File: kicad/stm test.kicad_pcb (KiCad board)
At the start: 2 copper layers, 2 parts, among them U101 MCP23008-xP

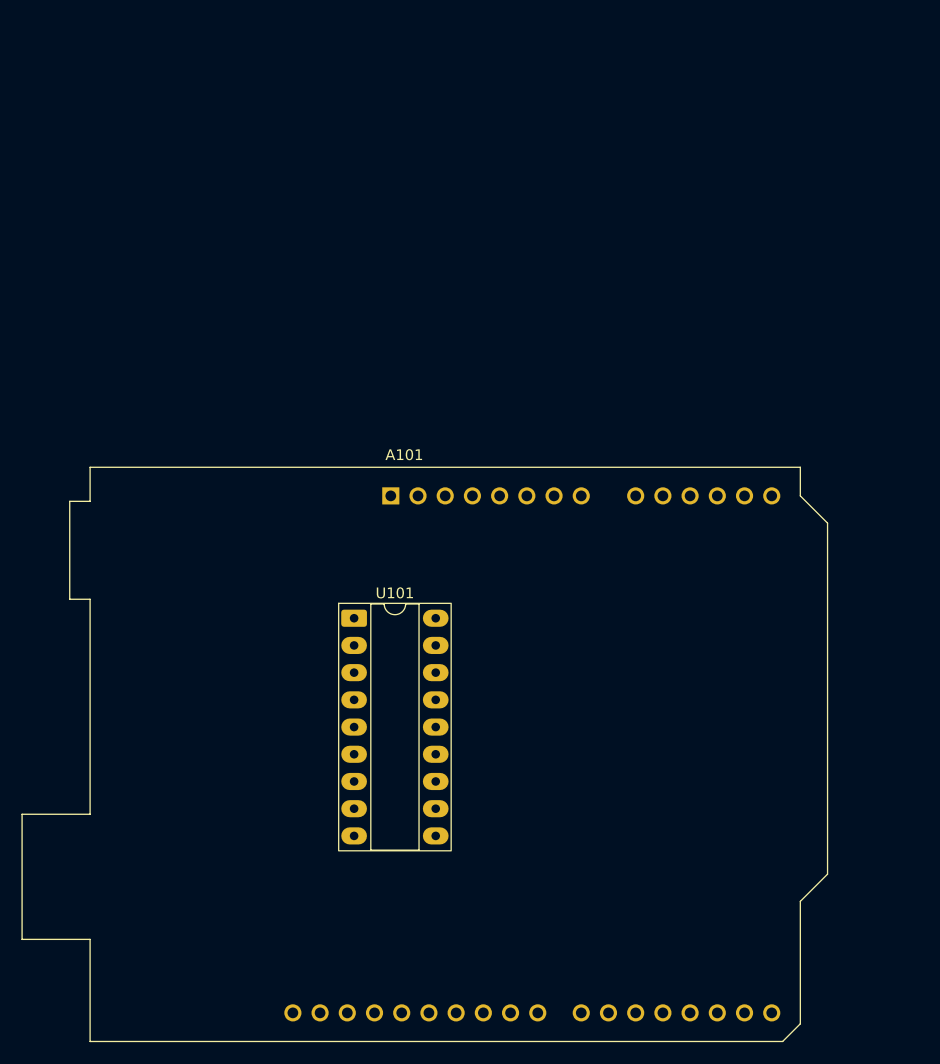
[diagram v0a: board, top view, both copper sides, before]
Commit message: i fugged up
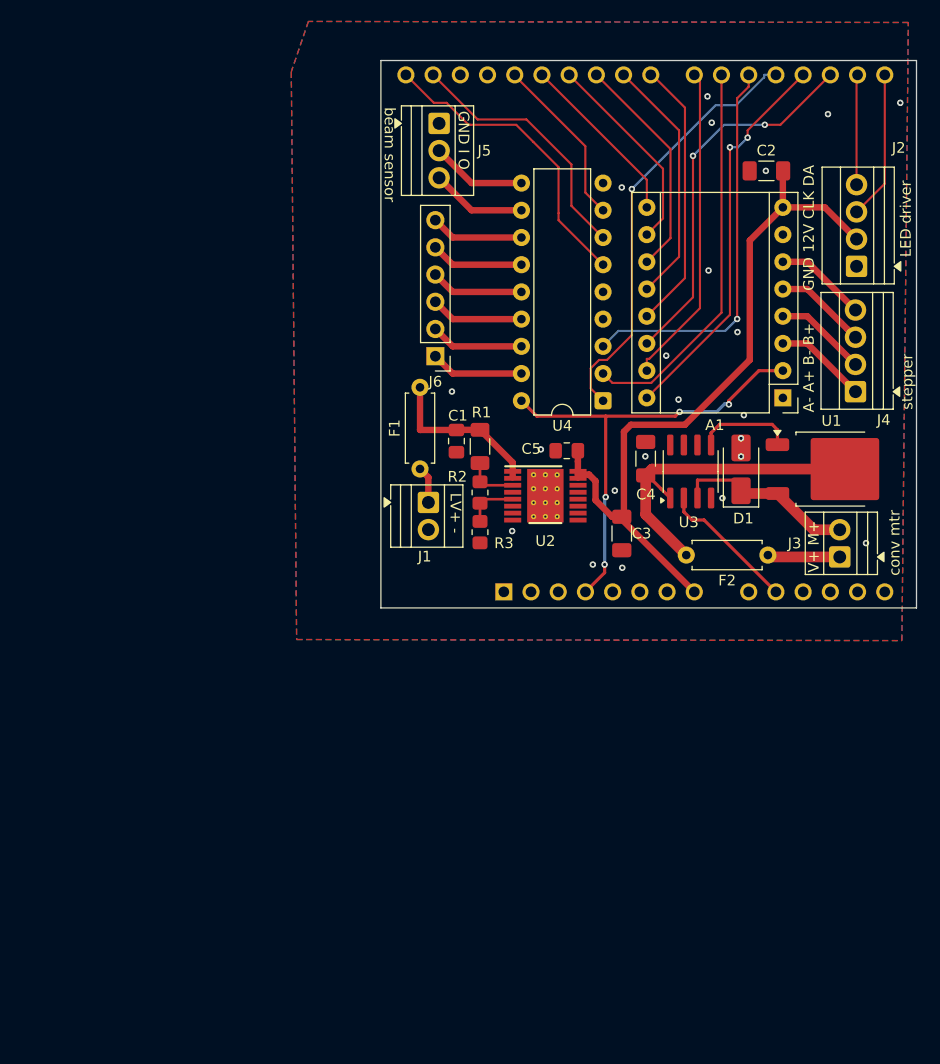
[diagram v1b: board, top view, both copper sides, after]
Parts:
- removed A101: Arduino_UNO_R3, Module:Arduino_UNO_R3
- removed U101: MCP23008-xP, Package_DIP:DIP-18_W7.62mm_Socket_LongPads
- added A1: Pololu_Breakout_A4988, Module:Pololu_Breakout-16_15.2x20.3mm, F.Cu at (158.0, 86.0)
- added A2: Arduino_UNO_R3, Module:Arduino_UNO_R3, B.Cu at (132.0, 104.1)
- added C1: 220n, Capacitor_SMD:C_0805_2012Metric_Pad1.18x1.45mm_HandSolder, F.Cu at (127.6, 90.0)
- added C2: 10u, Capacitor_SMD:C_1206_3216Metric_Pad1.33x1.80mm_HandSolder, F.Cu at (156.5, 64.8)
- added C3: 10u, Capacitor_SMD:C_1206_3216Metric_Pad1.33x1.80mm_HandSolder, F.Cu at (143.0, 98.7)
- added C4: 10u, Capacitor_SMD:C_1206_3216Metric_Pad1.33x1.80mm_HandSolder, F.Cu at (145.2, 91.7)
- added C5: 220n, Capacitor_SMD:C_0805_2012Metric_Pad1.18x1.45mm_HandSolder, F.Cu at (137.9, 90.9)
- added D1: ES1D, Diode_SMD:D_SMA, F.Cu at (154.1, 92.7)
- added F1: 1.5A, Resistor_THT:R_Axial_DIN0207_L6.3mm_D2.5mm_P7.62mm_Horizontal, F.Cu at (124.2, 92.6)
- added F2: 1.5A, Resistor_THT:R_Axial_DIN0207_L6.3mm_D2.5mm_P7.62mm_Horizontal, F.Cu at (156.6, 100.7)
- added J1: pwr, TerminalBlock:TerminalBlock_Xinya_XY308-2.54-2P_1x02_P2.54mm_Horizontal, F.Cu at (125.0, 95.8)
- added J2: led_driver, TerminalBlock:TerminalBlock_Xinya_XY308-2.54-4P_1x04_P2.54mm_Horizontal, F.Cu at (164.9, 73.7)
- added J3: conv motor, TerminalBlock:TerminalBlock_Xinya_XY308-2.54-2P_1x02_P2.54mm_Horizontal, F.Cu at (163.3, 100.8)
- added J4: stepper, TerminalBlock:TerminalBlock_Xinya_XY308-2.54-4P_1x04_P2.54mm_Horizontal, F.Cu at (164.8, 85.4)
- added J5: beam sensor, TerminalBlock:TerminalBlock_Xinya_XY308-2.54-3P_1x03_P2.54mm_Horizontal, F.Cu at (126.0, 60.4)
- added J6: Conn_01x06_Pin, Connector_PinHeader_2.54mm:PinHeader_1x06_P2.54mm_Vertical, F.Cu at (125.6, 82.1)
- added R1: 432k, Resistor_SMD:R_1206_3216Metric_Pad1.30x1.75mm_HandSolder, F.Cu at (129.8, 90.5)
- added R2: 38.3k, Resistor_SMD:R_0805_2012Metric_Pad1.20x1.40mm_HandSolder, F.Cu at (129.8, 94.8)
- added R3: 49.9k, Resistor_SMD:R_0805_2012Metric_Pad1.20x1.40mm_HandSolder, F.Cu at (129.8, 98.5)
- added U1: IPD14N06, Package_TO_SOT_SMD:TO-252-2, F.Cu at (162.6, 92.6)
- added U2: TPS26600PWPR, local:PWP0016H_M, F.Cu at (135.9, 95.1)
- added U3: MIC5014YM, Package_SO:SOIC-8_3.9x4.9mm_P1.27mm, F.Cu at (149.4, 92.9)
- added U4: MCP23S08-xP, Package_DIP:DIP-18_W7.62mm, F.Cu at (141.3, 86.3)
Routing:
- net +12V: track 0.00 -> 69.7 mm
- net +3V3: track 0.00 -> 44.2 mm, vias 0 -> 4
- net /spiA.sclk: track 0.00 -> 40.3 mm, vias 0 -> 1
- net /spiA.miso: track 0.00 -> 36.8 mm, vias 0 -> 1
- net /stepper.dir: track 0.00 -> 36.6 mm, vias 0 -> 2
- net /spiA.mosi: track 0.00 -> 36.3 mm
- net /stepper.sleep_n: track 0.00 -> 35.2 mm, vias 0 -> 2
- net Net-(U1-D): track 0.00 -> 32.2 mm
- net /stepper.step: track 0.00 -> 30.0 mm
- net /mcp.rst_n: track 0.00 -> 28.6 mm
- net /stepper.reset_n: track 0.00 -> 25.4 mm
- net /spiA.cs_MCP: track 0.00 -> 24.4 mm
- net /stepper.ms3: track 0.00 -> 23.4 mm
- net /stepper.ms2: track 0.00 -> 21.2 mm
- net /stepper.ms1: track 0.00 -> 19.2 mm
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- added copper zone on B.Cu, net GND
- added copper zone on F.Cu, net GND
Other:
- board outline added: 50 x 51.1 mm
- board text added: "A- A+ B- B+"
- board text added: "GND 12V CLK DA"
- board text added: "GND I O"
- board text added: "LED driver"
- board text added: "LV+ -"
- board text added: "V+ M+"
- board text added: "beam sensor"
- board text added: "conv mtr"
- board text added: "stepper"
